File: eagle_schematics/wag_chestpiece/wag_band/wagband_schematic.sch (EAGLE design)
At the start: 8 parts, among them U2 TLV1117-33CDCY

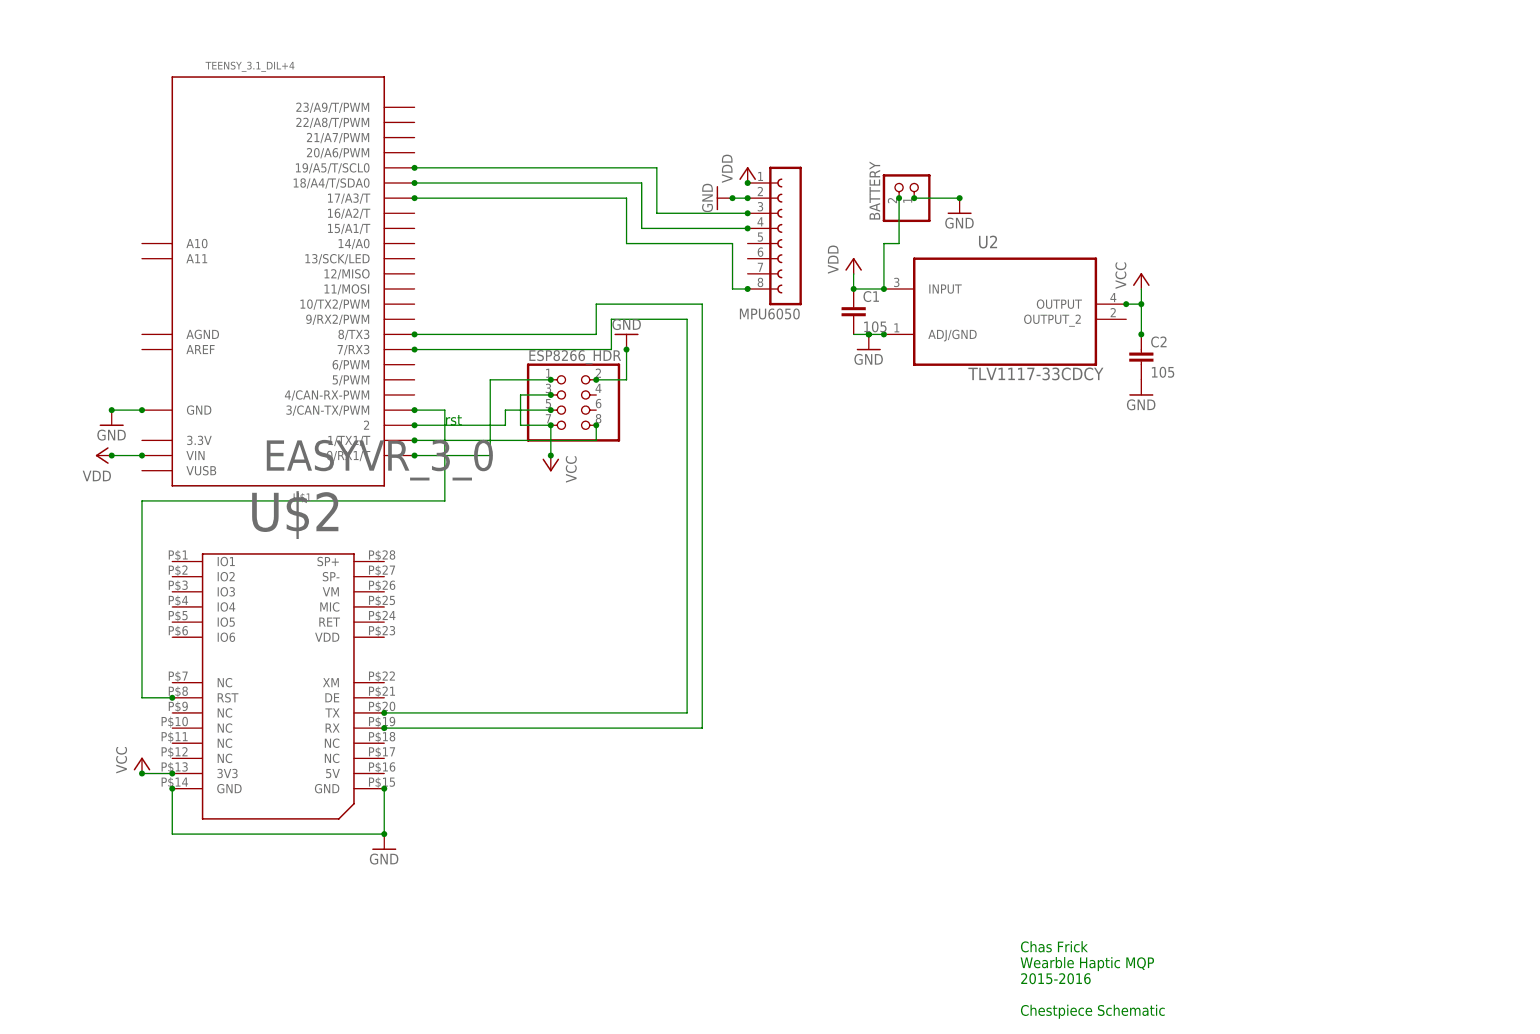
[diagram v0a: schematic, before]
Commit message: Added more parts for eagle
Finished PCBs
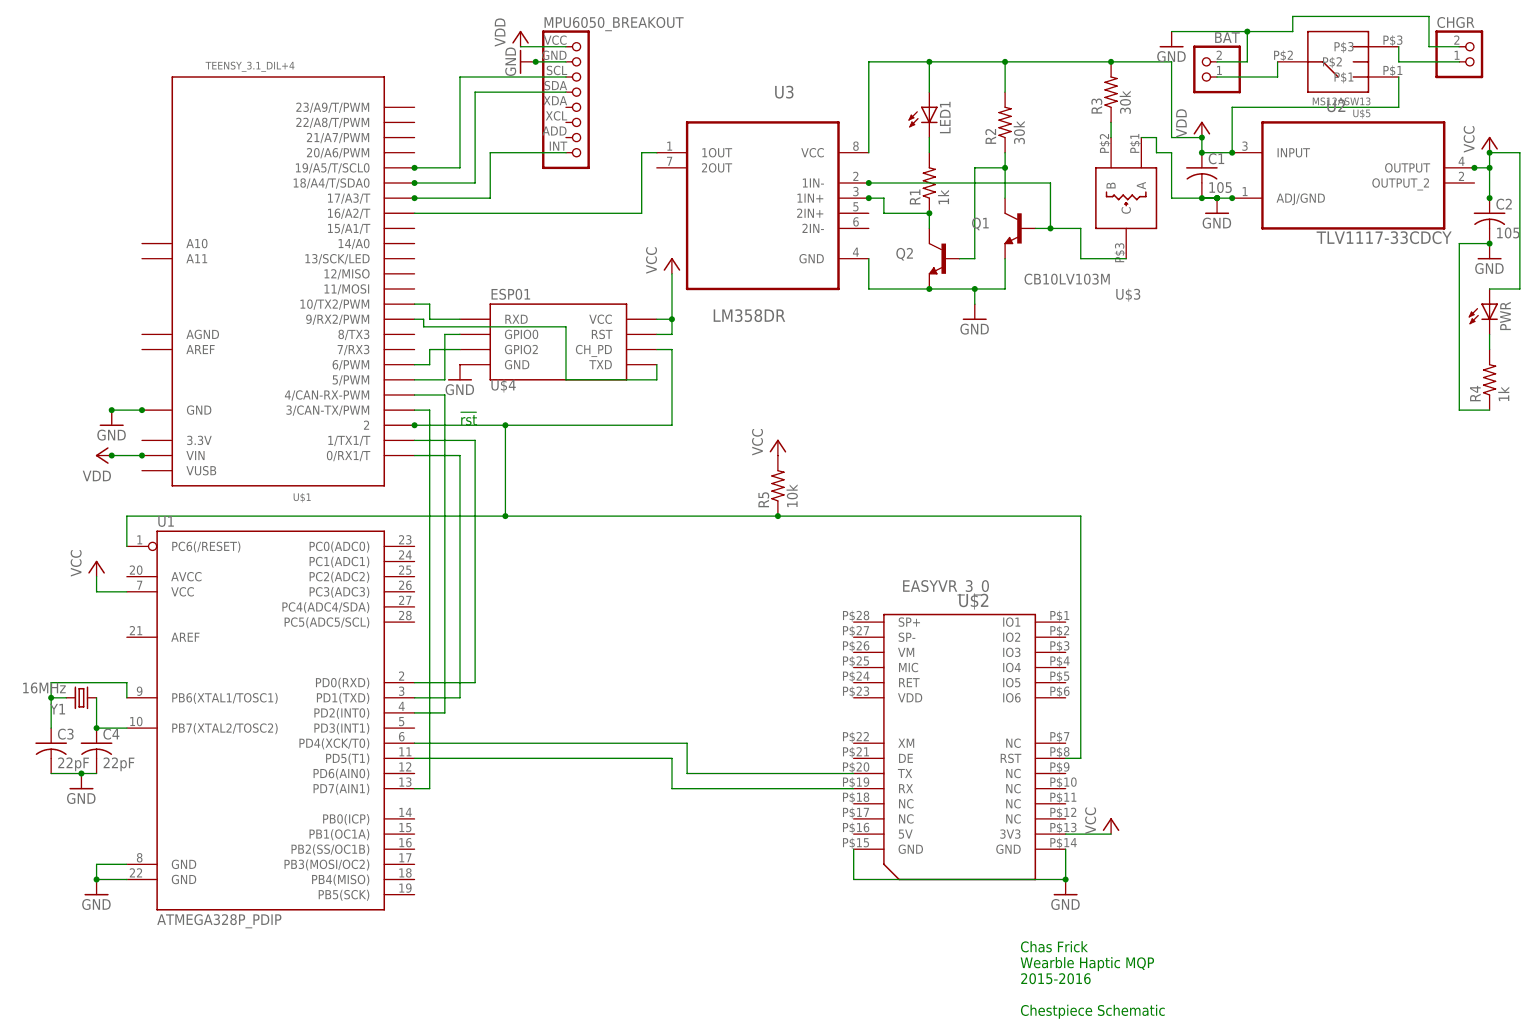
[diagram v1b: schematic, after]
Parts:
- removed BATTERY: (no value), adafruit:JST_2PIN-THM-RA
- removed ESP8266_HDR: (no value), pinhead:PINHD-2X4
- removed MPU6050: (no value), con-lsta:FE08-1
- added BAT, CHGR: (no value), adafruit:JST_2PIN-THM-RA
- added C3, C4: 22pF, rcl:C-USC1206K
- added LED1, PWR: (no value), led:LED5MM
- added MPU6050_BREAKOUT: (no value), mqp_custom_parts:MPU6050_BREAKOUT
- added Q1, Q2: (no value), mqp_custom_parts:TRANSISTOR_NPNMMBT3904
- added R1, R4: 1k, resistor:R-US_R1206
- added R2, R3: 30k, resistor:R-US_R1206
- added R5: 10k, resistor:R-US_R1206
- added U$3: CB10LV103M, mqp_custom_parts:CB10LV103M
- added U$4: ESP01, esp8266modules:ESP01
- added U$5: MS12ASW13, mqp_custom_parts:MS12ASW13
- added U1: ATMEGA328P_PDIP, SparkFun-DigitalIC:ATMEGA328P_PDIP
- added U3: LM358DR, Texas Instruments_By_element14_Batch_1:LM358DR
- added Y1: 16MHz, SparkFun-FreqCtrl:CRYSTALSMD
- C1, C2: device rcl:C-EU025-024X044 -> resistor:C-USC0805K
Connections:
- new net !RST: R5.1, U$1.2, U$2.RST, U$4.CH_PD, U1.PC6(/RESET)
- new net N$10: Q2.C, R1.1, U3.1IN+
- new net N$11: R3.1, U$3.B
- new net N$12: LED1.C, R1.2
- new net N$13: U$1.1/TX1/T, U1.PD0(RXD)
- new net N$14: U$1.16/A2/T, U3.1OUT
- new net N$15: PWR.C, R4.2
- new net N$16: U$1.3/CAN-TX/PWM, U1.PD7(AIN1)
- new net N$18: U$1.6/PWM, U$4.GPIO2
- new net N$20: C3.1, U1.PB6(XTAL1/TOSC1), Y1.2
- new net N$22: U$1.0/RX1/T, U1.PD1(TXD)
- new net N$23: BAT.2, U$5.P$2
- new net N$25: CHGR.2, U$5.P$3
- new net N$3: MPU6050_BREAKOUT.SDA, U$1.18/A4/T/SDA0
- new net N$6: U$2.TX, U1.PD4(XCK/T0)
- new net N$9: Q1.C, Q2.B, R2.1
- net GND: now also BAT.1, C3.2, C4.2, CHGR.1, MPU6050_BREAKOUT.GND, Q1.E, Q2.E, R4.1, U$3.A, U$4.GND, U1.GND@1, U1.GND@2, U3.GND; no longer BATTERY.2, ESP8266_HDR.2, MPU6050.2
- net N$1: now also U$1.4/CAN-RX-PWM, U1.PD2(INT0); no longer U$1.7/RX3, U$2.TX
- net N$17: now also MPU6050_BREAKOUT.SCL; no longer MPU6050.3
- net N$19: now also U$1.9/RX2/PWM, U$4.TXD; no longer ESP8266_HDR.8, U$1.1/TX1/T
- net N$2: now also U$1.10/TX2/PWM, U$4.RXD; no longer U$1.8/TX3, U$2.RX
- net N$21: now also C4.1, U1.PB7(XTAL2/TOSC2), Y1.1; no longer ESP8266_HDR.5, U$1.2
- net N$4: now also Q1.B, U$3.C, U3.1IN-; no longer MPU6050.4, U$1.18/A4/T/SDA0
- net N$5: now also U$2.RX, U1.PD5(T1); no longer U$1.3/CAN-TX/PWM, U$2.RST
- net N$7: now also U$1.5/PWM, U$4.GPIO0; no longer ESP8266_HDR.1, U$1.0/RX1/T
- net N$8: now also MPU6050_BREAKOUT.INT; no longer MPU6050.8
- net VCC: now also LED1.A, MPU6050_BREAKOUT.VCC, PWR.A, R2.2, R3.2, R5.2, U$4.RST, U$4.VCC, U$5.P$1, U1.VCC, U3.VCC; no longer BATTERY.1, ESP8266_HDR.3, ESP8266_HDR.7, MPU6050.1
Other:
- note added: "!rst"
- note removed: "rst"
- moved on the sheet: C1, C2, U$2, U2
